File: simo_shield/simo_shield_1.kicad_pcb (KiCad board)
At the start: 2 copper layers, 64.6 x 82.5 mm, 6 parts, among them J1 CONECTOR DEBUG_UART, U1 YAAJ_BluePill_Part_Like_SWD_B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, U2 elemon_board, U3 flash_externa, U4 mpu6050

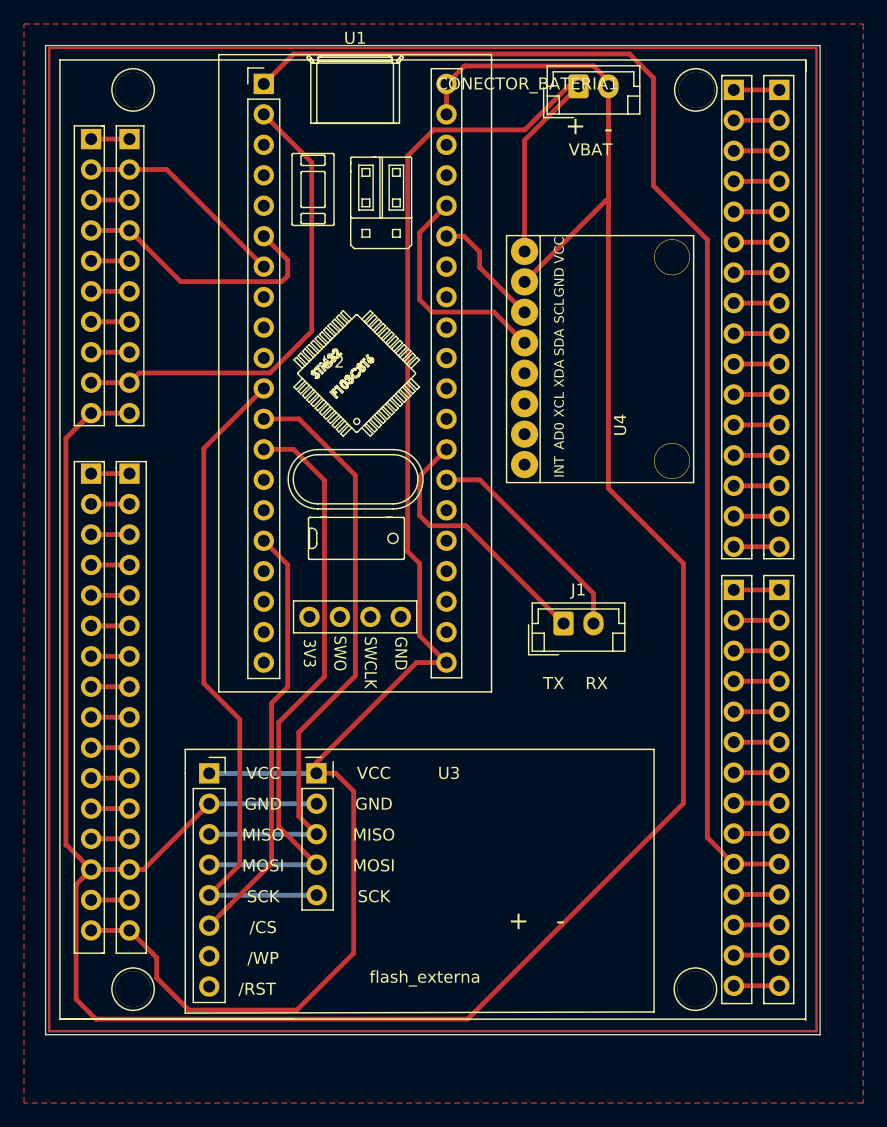
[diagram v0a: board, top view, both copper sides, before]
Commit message: update en pcb shield
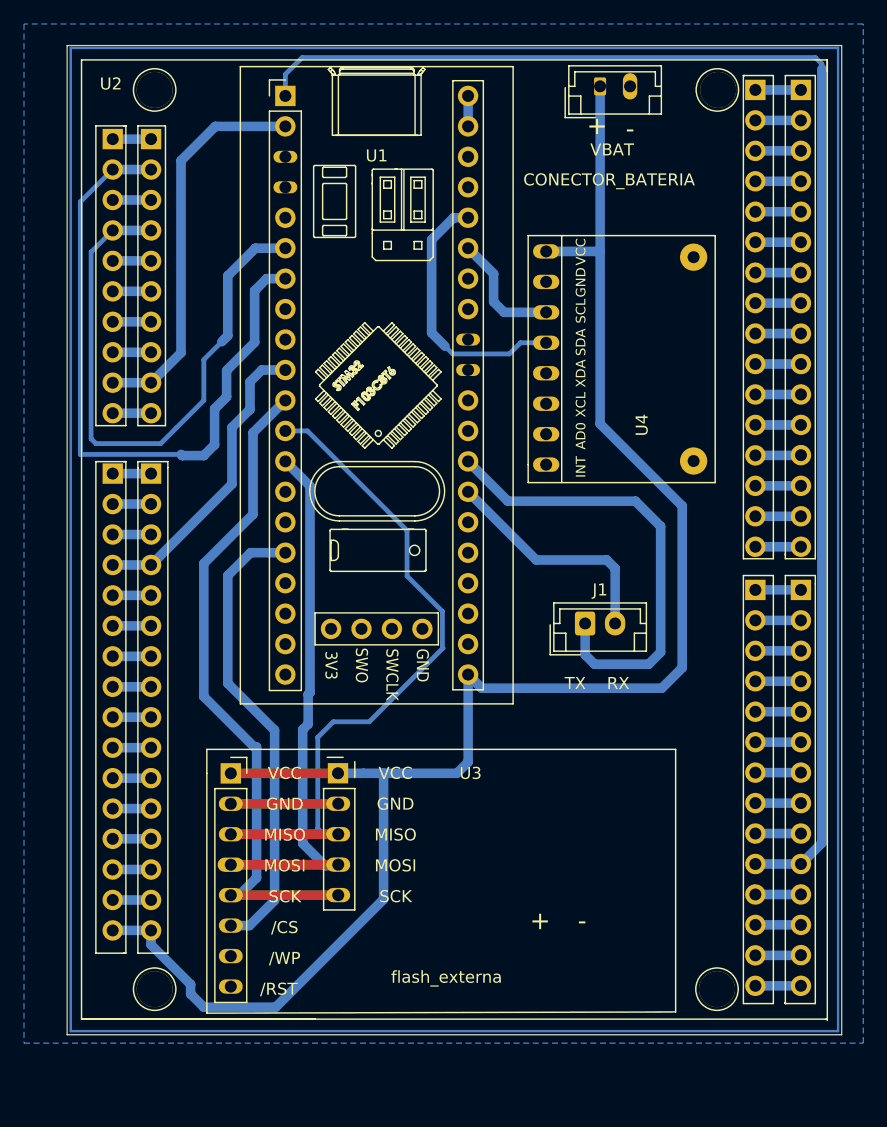
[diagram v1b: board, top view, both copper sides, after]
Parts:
- moved U1 2.06 mm to (66.8, 71.0)
- moved CONECTOR_BATERIA 1.80 mm to (93.0, 70.2)
- moved J1 1.80 mm to (91.8, 115.0)
- moved U2 1.80 mm to (49.8, 68.0)
- moved U3 1.80 mm to (62.2, 127.5)
- moved U4 1.80 mm to (88.5, 101.8)
- renumbered CONECTOR_BATERIA1 to CONECTOR_BATERIA
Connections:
- U1 pad 10: unconnected-(U1-Pad10) -> Net-(U2-Pad14)
- U2 pad 14: unconnected-(U2-Pad14) -> Net-(U2-Pad14)
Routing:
- net /BAT_GND: track 224.1 -> 17.9 mm
- net Net-(U1-Pad7): track 17.8 -> 56.9 mm
- net Net-(U1-Pad6): track 22.5 -> 49.4 mm
- net Net-(U2-Pad14): track 0.00 -> 25.2 mm
- net Net-(J1-Pad1): track 22.2 -> 38.5 mm
- net /BAT_ENA_PIN: track 106.5 -> 118.6 mm
- net Net-(U1-Pad2): track 39.9 -> 32.6 mm
- net Net-(U1-Pad12): track 51.1 -> 56.6 mm
- net Net-(U1-Pad13): track 50.0 -> 45.7 mm
- net Net-(U1-Pad36): track 19.0 -> 22.2 mm
- net unconnected-(U2-Pad14): track 3.20 -> 0.00 mm
- net Net-(U1-Pad16): track 35.6 -> 38.8 mm
- net +BATT: track 144.9 -> 143.0 mm
- net Net-(J1-Pad2): track 18.7 -> 19.5 mm
- net Net-(U1-Pad11): track 55.6 -> 56.3 mm
- added copper zone on B.Cu, net /BAT_GND
- removed copper zone on F.Cu, net /BAT_GND
